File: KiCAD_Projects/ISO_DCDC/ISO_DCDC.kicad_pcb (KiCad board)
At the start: 2 copper layers, 90 x 100 mm, 81 parts, among them IC1 PC817, IC2 PC817, IC3 PC817, IC4 PC817, IC5 PC817, P1 CONN_01X01, P10 CONN_01X02, P11 CONN_01X02, P12 CONN_01X01, P13 CONN_01X04, P14 CONN_01X02, P15 CONN_01X02, P19 CONN_01X01, P2 CONN_01X01, P20 CONN_01X01, P21 CONN_01X02, P22 CONN_01X01, P23 CONN_01X01, P25 CONN_01X01, P26 CONN_01X01, P3 CONN_01X01, P4 CONN_01X02, P5 CONN_01X02, P6 CONN_01X04, P7 CONN_01X04, P8 CONN_01X01, P9 CONN_01X01, Q1 MOSFET_N, U1 V23076-D3001-D142, U2 V23076-D3001-D142, U3 V23076-D3001-D142

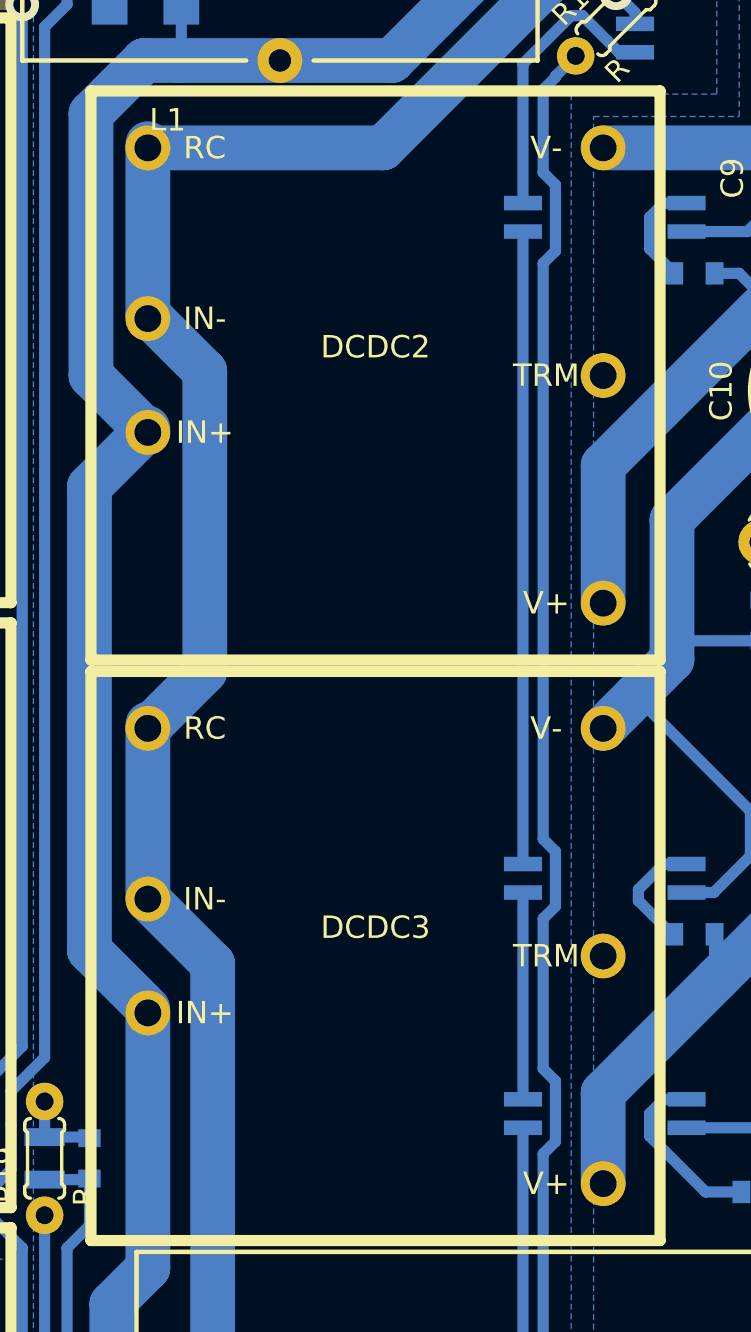
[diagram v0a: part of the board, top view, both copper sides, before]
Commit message: 3Dデータ組み合わてテスト
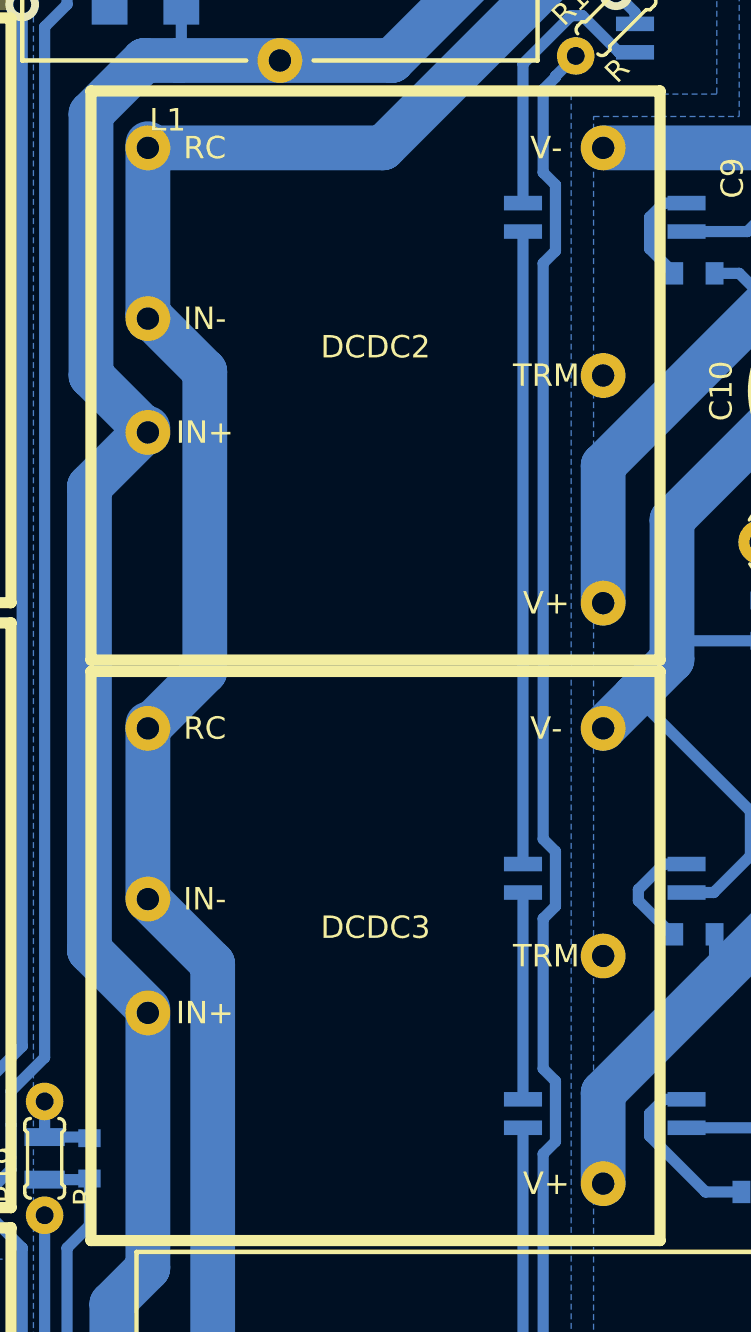
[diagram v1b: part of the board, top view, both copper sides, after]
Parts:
- DCDC4: footprint RP_KiCAD_Libs:MGS30 -> Converters_DCDC_ACDC:MGS30
